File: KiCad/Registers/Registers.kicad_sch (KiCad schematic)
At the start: 29 parts, among them J1 TO_BACKPLANE, J2 ACCUMULATOR_OUT, J3 FROM_CTRL, J4 TO_MEMORY, J5 TO_FP, U31 74HC74, U32 74HCT32, U37 74HC688, U38 74HC688, U39 74HC688, U40 74HC688, U46 74HC244, U47 74HC244, U48 74HC244, U50 74AHC1G04

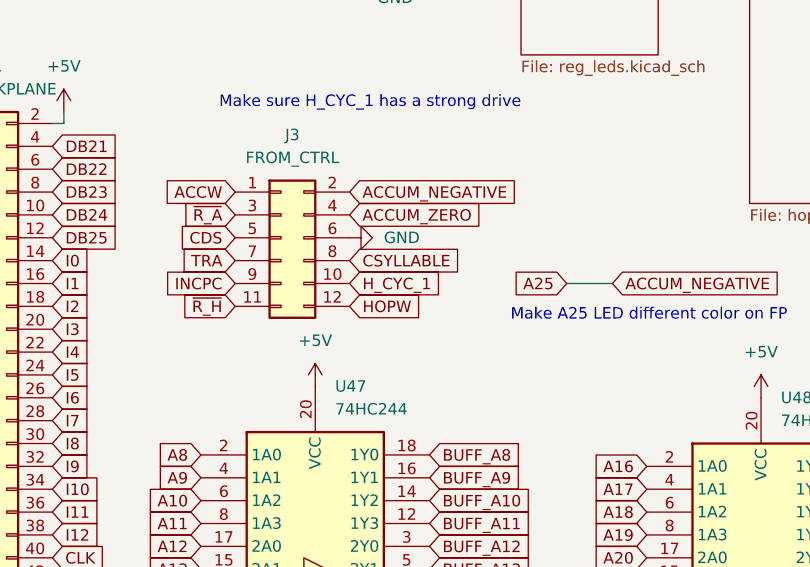
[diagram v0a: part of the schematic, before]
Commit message: Update schematics with fixes.
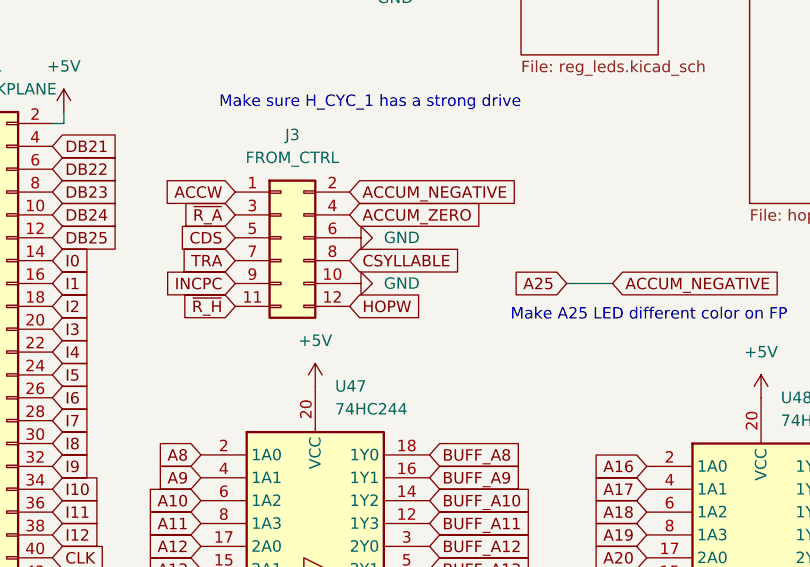
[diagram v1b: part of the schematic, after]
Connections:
- net H_CYC_1 is gone; now on net GND: J3.10 (Pin_10)
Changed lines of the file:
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@@
 		)
 	)
-	(global_label "H_CYC_1"
-		(shape input)
-		(at 82.55 101.6 0)
-		(fields_autoplaced yes)
-		(effects
-			(font
-				(size 1.27 1.27)
-			)
-			(justify left)
-		)
-		(property "Intersheetrefs" "${INTERSHEET_REFS}"
-			(at 93.639 101.6 0)
-			(effects
-				(font
-					(size 1.27 1.27)
-				)
-				(justify left)
-				(hide yes)
-			)
-		)
-	)
 	(global_label "DB9"
 		(shape input)
@@
 					(unit 1)
 				)
+			)
+		)
+	)
+	(symbol
+		(lib_id "power:GND")
+		(at 82.55 101.6 90)
+		(unit 1)
+		(exclude_from_sim no)
+		(in_bom yes)
+		(on_board yes)
+		(dnp no)
+		(fields_autoplaced yes)
+		(property "Reference" "#PWR0210"
+			(at 88.9 101.6 0)
+			(effects
+				(font
+					(size 1.27 1.27)
+				)
+				(hide yes)
+			)
+		)
+		(property "Value" "GND"
+			(at 86.36 101.5999 90)
+			(effects
+				(font
+					(size 1.27 1.27)
+				)
+				(justify right)
+			)
+		)
+		(property "Footprint" ""
+			(at 82.55 101.6 0)
+			(effects
+				(font
+					(size 1.27 1.27)
+				)
+				(hide yes)
+			)
+		)
+		(property "Datasheet" ""
+			(at 82.55 101.6 0)
+			(effects
+				(font
+					(size 1.27 1.27)
+				)
+				(hide yes)
+			)
+		)
+		(property "Description" "Power symbol creates a global label with name \"GND\" , ground"
+			(at 82.55 101.6 0)
+			(effects
+				(font
+					(size 1.27 1.27)
+				)
+				(hide yes)
+			)
+		)
+		(pin "1"
+		)
+		(instances
+			(project "Registers"
+				(path "/bb2d8093-1baa-42e1-9f61-d1b3316cfdc8"
+					(reference "#PWR0210")
+					(unit 1)
+				)
